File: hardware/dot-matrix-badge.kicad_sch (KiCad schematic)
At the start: 15 parts, among them J1 AVR-UPDI-6, J2 JST_04, SW1 SW_SPST, SW2 SW_Push, SW3 SW_Push, U1 ATtiny1604-SS

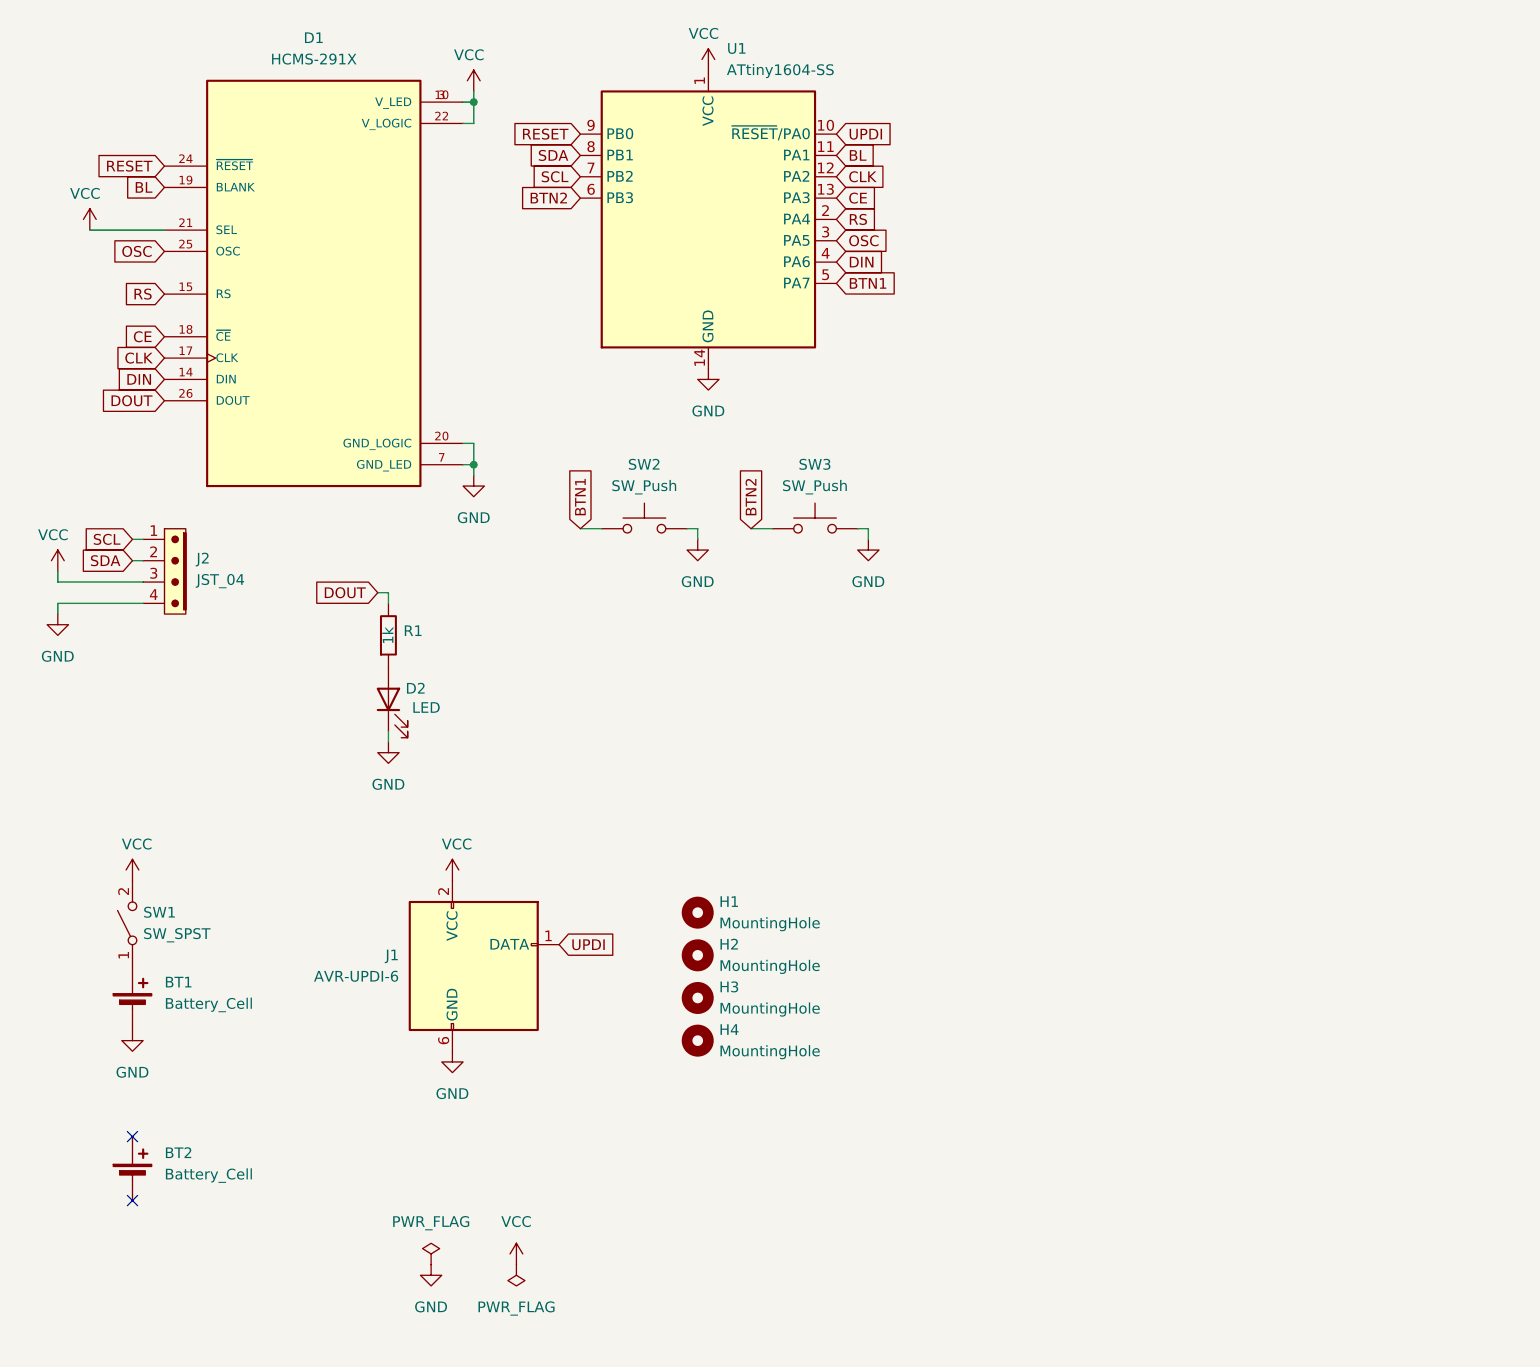
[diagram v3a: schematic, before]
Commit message: 99% done
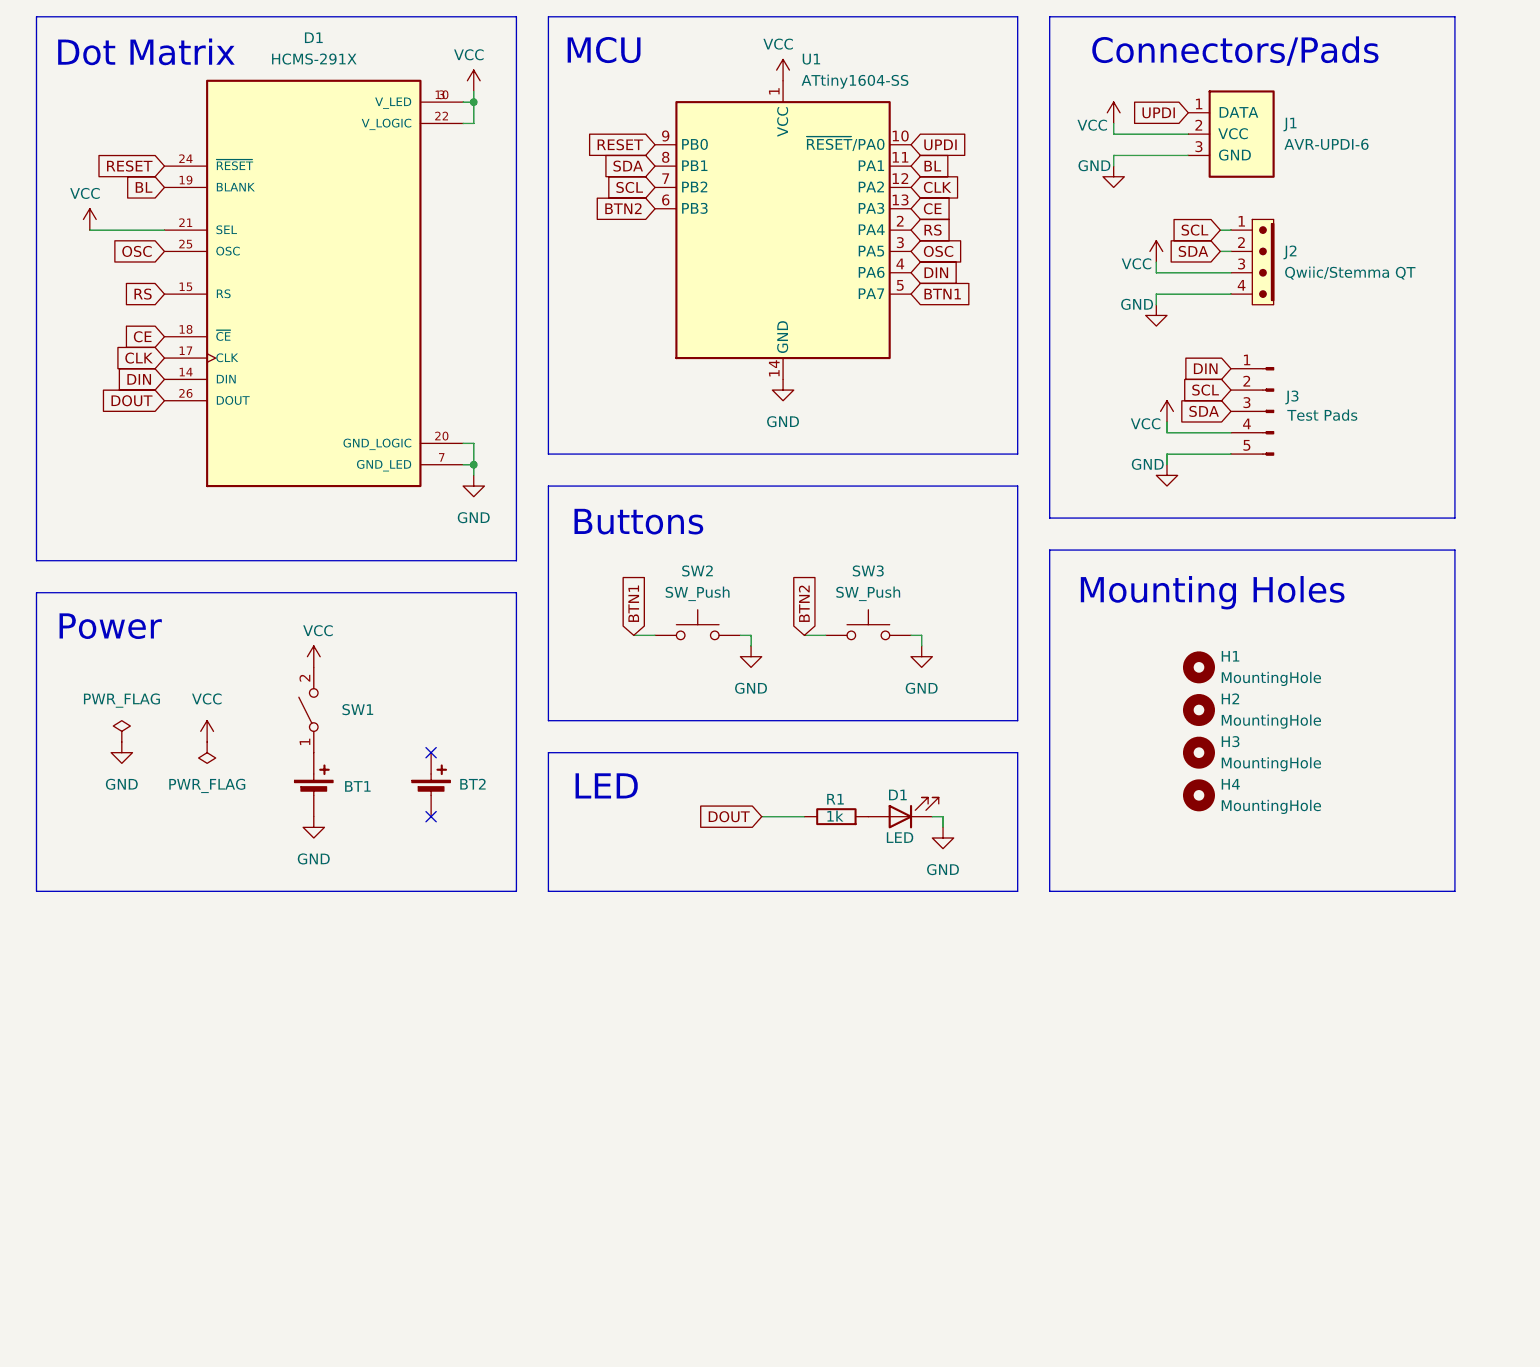
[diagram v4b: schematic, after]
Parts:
- added J3: Test Pads, symbol Connector:Conn_01x05_Pin
- J1: symbol Connector:AVR-UPDI-6 -> DotMatrixBadge:AVR-UPDI-3
- J2: value JST_04 -> Qwiic/Stemma QT
- R1: footprint Resistor_SMD:R_0402_1005Metric -> Resistor_SMD:R_0603_1608Metric
- renumbered D2 to D1
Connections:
- net DIN: now also J3.1 (Pin_1)
- net GND: now also J1.3 (GND), J3.5 (Pin_5); no longer J1.6 (GND)
- net SCL: now also J3.2 (Pin_2)
- net SDA: now also J3.3 (Pin_3)
- net VCC: now also J3.4 (Pin_4)
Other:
- note added: "Buttons"
- note added: "Connectors/Pads"
- note added: "Dot Matrix"
- note added: "LED"
- note added: "MCU"
- note added: "Mounting Holes"
- note added: "Power"
- title: (none) -> Dot Matrix Badge
- moved on the sheet: BT1, BT2, D1, H1, H2, H3, H4, J2, R1, SW1, SW2, SW3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
